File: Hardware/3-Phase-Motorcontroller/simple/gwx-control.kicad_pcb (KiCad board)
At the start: 2 copper layers, 54 x 33 mm, 39 parts, among them J10 Conn_02x08_Odd_Even, T1 BC850, T2 BC850, U1 74LS02, U2 74LS123

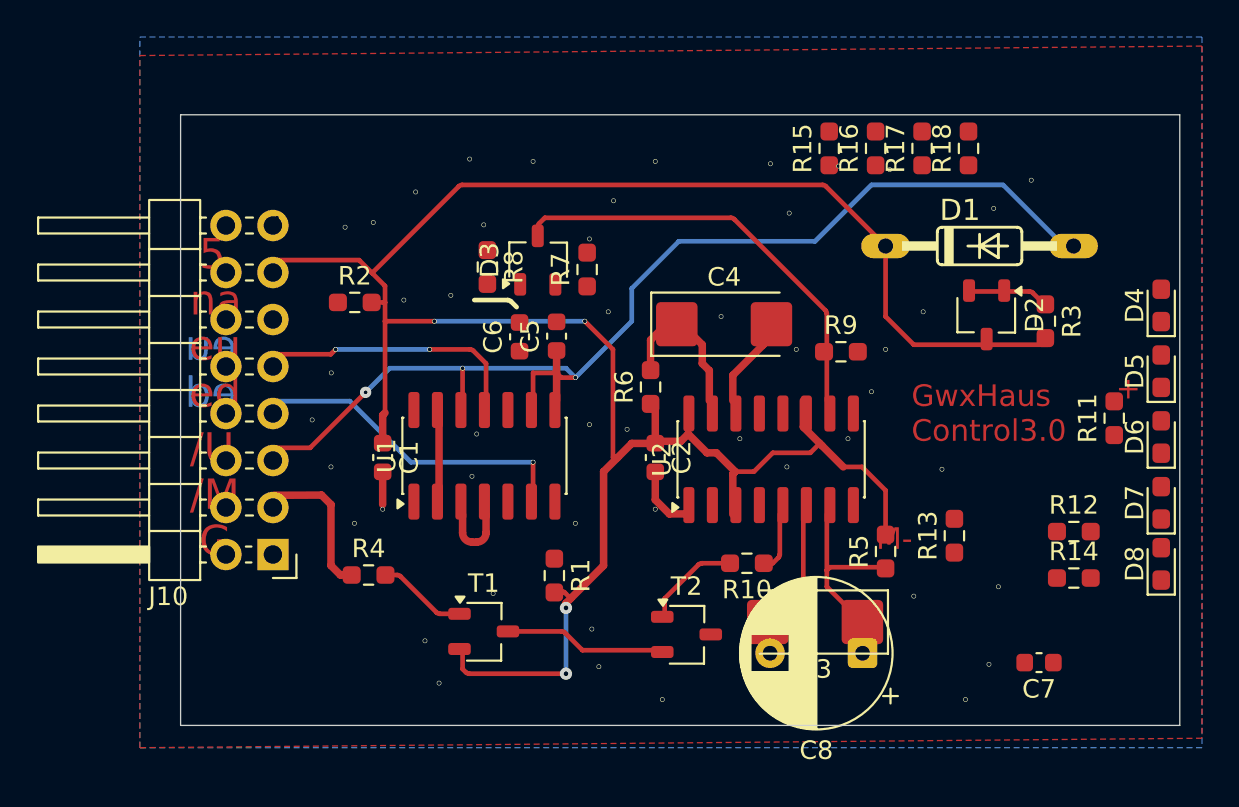
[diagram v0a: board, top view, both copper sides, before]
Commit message: PCB shrinked
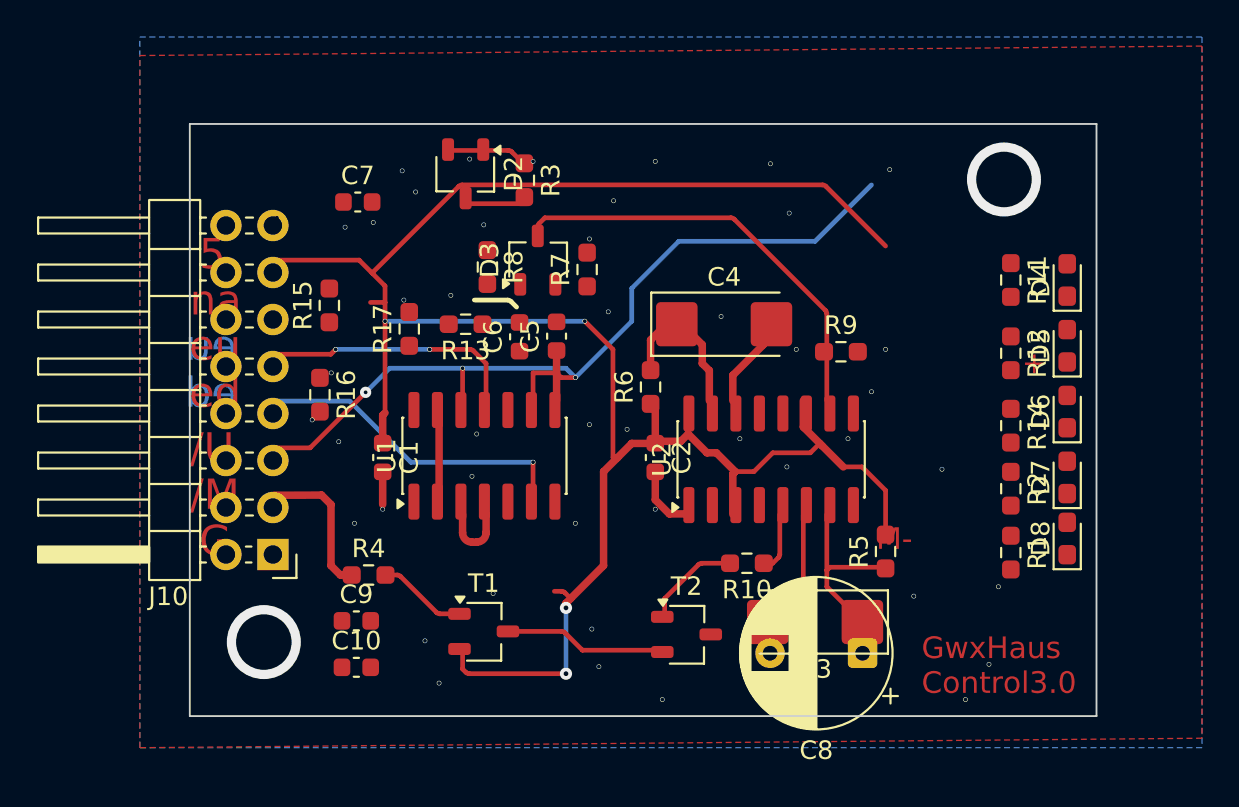
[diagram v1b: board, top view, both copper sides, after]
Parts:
- removed D1: 1N4148, DO35-10
- removed R18: 4k7, Resistor_SMD:R_0603_1608Metric_Pad0.98x0.95mm_HandSolder
- added C10: 100n, Capacitor_SMD:C_0603_1608Metric, F.Cu at (131.0, 118.4)
- added C9: 100n, Capacitor_SMD:C_0603_1608Metric, F.Cu at (131.0, 115.9)
- moved C7 44.4 mm to (131.1, 93.2), turned to 0 degrees
- moved R2 36.9 mm to (166.4, 108.7), turned to -90 degrees
- moved R16 32.8 mm to (129.0, 103.6), turned to -90 degrees
- moved R17 29.4 mm to (133.9, 100.1)
- moved R3 29.2 mm to (140.1, 92.0)
- moved D2 29.2 mm to (136.9, 91.7)
- moved R13 28.8 mm to (136.9, 99.8), turned to 180 degrees
- moved R15 28.3 mm to (129.5, 98.8)
- moved R1 24.7 mm to (166.4, 112.2)
- moved R12 10.2 mm to (166.4, 101.4), turned to -90 degrees
- moved R11 9.33 mm to (166.4, 97.4), turned to -90 degrees
- moved R14 8.91 mm to (166.4, 105.3), turned to -90 degrees
- moved D6 5.26 mm to (169.4, 104.5)
- moved D7 5.26 mm to (169.4, 108.1)
- moved D4 5.26 mm to (169.4, 97.4)
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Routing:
- net //UP: track 64.1 -> 52.3 mm, vias 3 -> 4
- net VCC: track 128.1 -> 118.1 mm
- net Net-(J10-Pin_7): vias 1 -> 2
- net GND: vias 46 -> 44
- net //END_UP: vias 1 -> 0
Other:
- board size 54 x 33 mm -> 49 x 32 mm
